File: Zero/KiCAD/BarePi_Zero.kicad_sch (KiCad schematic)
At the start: 2 parts, among them J1 Raspberry_Pi_Zero, J2 OUT

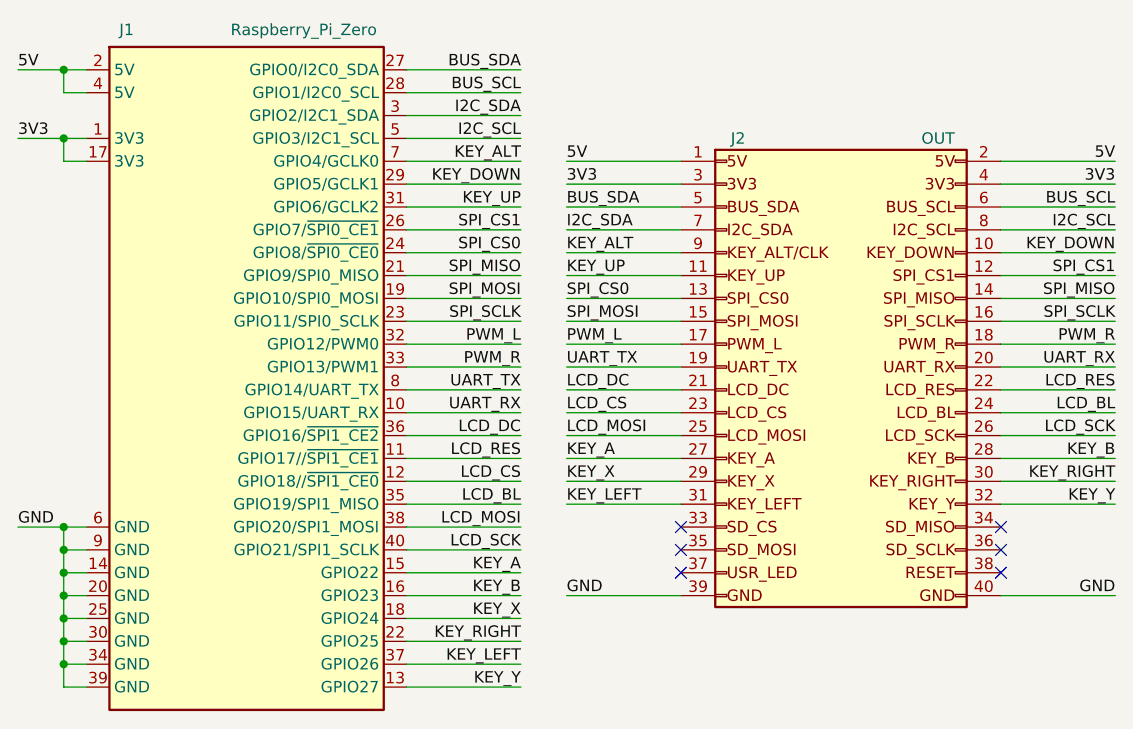
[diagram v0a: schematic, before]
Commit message: init
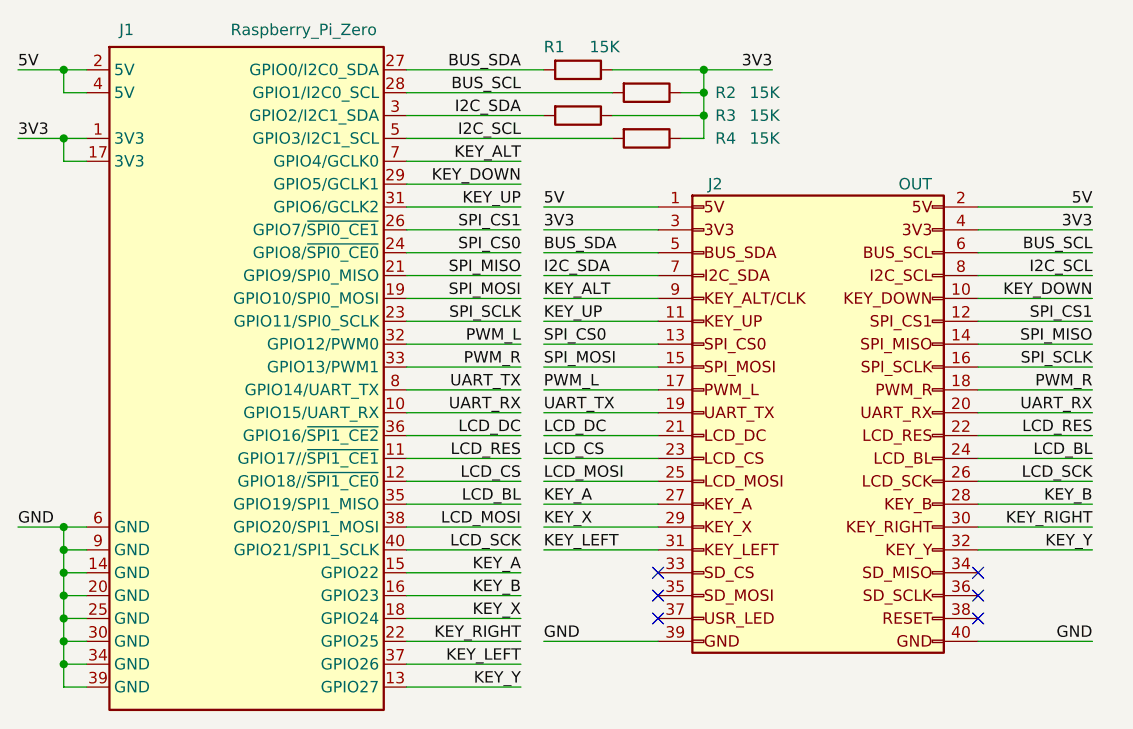
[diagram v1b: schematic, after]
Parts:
- added R1, R2, R3, R4: 15K, Resistor_SMD:R_1206_3216Metric_Pad1.30x1.75mm_HandSolder, symbol Device:R
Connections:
- net 3V3: now also R1.1, R2.1, R3.1, R4.1
- net BUS_SCL: now also R2.2
- net BUS_SDA: now also R1.2
- net I2C_SCL: now also R4.2
- net I2C_SDA: now also R3.2
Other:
- moved on the sheet: J2
